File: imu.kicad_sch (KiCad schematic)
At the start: 5 parts, among them U2 MPU-6000

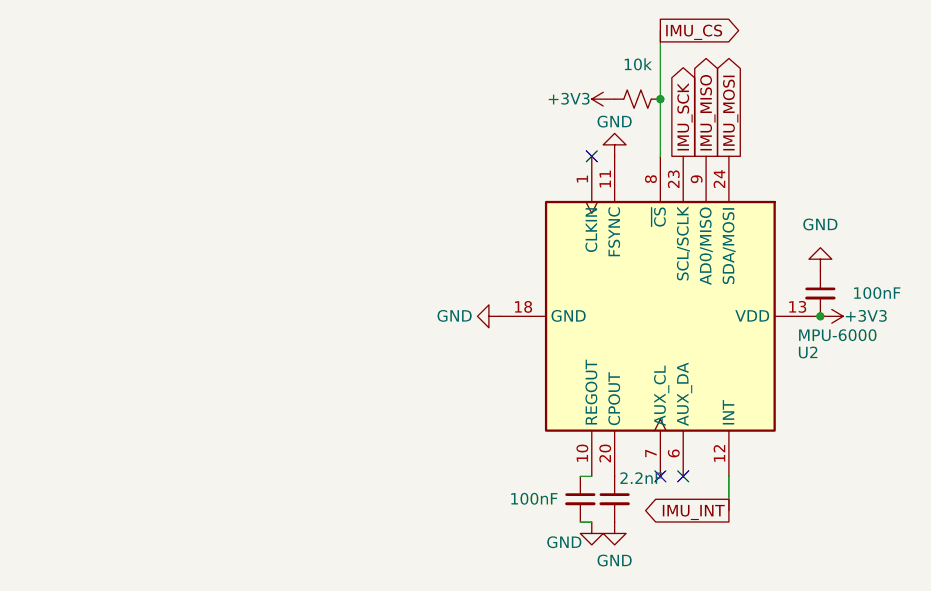
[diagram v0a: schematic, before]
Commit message: done?
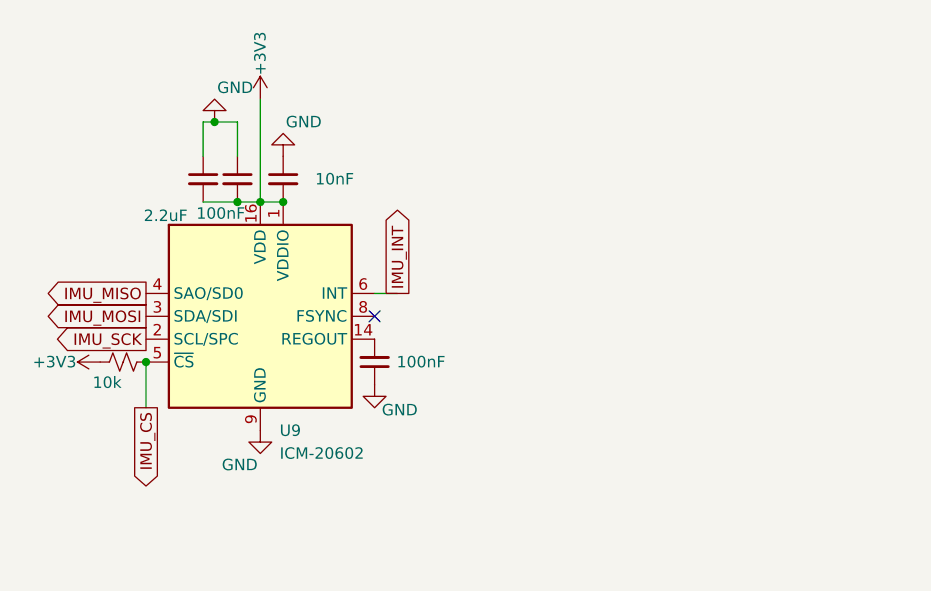
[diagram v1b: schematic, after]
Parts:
- removed C9: 2.2nF, Capacitor_SMD:C_0603_1608Metric_Pad1.08x0.95mm_HandSolder, symbol Device:C_Small
- removed U2: MPU-6000, Sensor_Motion:InvenSense_QFN-24_4x4mm_P0.5mm, symbol Sensor_Motion:MPU-6000
- added C44: 10nF, Capacitor_SMD:C_0603_1608Metric_Pad1.08x0.95mm_HandSolder, symbol Device:C_Small
- added C45: 2.2uF, Capacitor_SMD:C_0603_1608Metric_Pad1.08x0.95mm_HandSolder, symbol Device:C_Small
- added U9: ICM-20602, Package_LGA:LGA-16_3x3mm_P0.5mm, symbol Sensor_Motion:ICM-20602
- R3: footprint Resistor_SMD:R_0603_1608Metric_Pad0.98x0.95mm_HandSolder -> Resistor_SMD:R_0402_1005Metric_Pad0.72x0.64mm_HandSolder
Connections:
- net +3V3: now also C44.2, C45.2, U9.1 (VDDIO), U9.16 (VDD)
- net GND: now also C7.1, C44.1, C45.1, U9.10 (GND), U9.11 (GND), U9.12 (GND), U9.13 (GND), U9.15 (GND), U9.9 (GND); no longer C7.2
- net IMU_CS: now also U9.5 (~{CS})
- net IMU_INT: now also U9.6 (INT)
- net IMU_MISO: now also U9.4 (SAO/SD0)
- net IMU_MOSI: now also U9.3 (SDA/SDI)
- net IMU_SCK: now also U9.2 (SCL/SPC)
- new net: C7.2, U9.14 (REGOUT)
- no-connect marks 3 -> 1
